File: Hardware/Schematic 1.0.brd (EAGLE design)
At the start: 119.4 x 63.5 mm, 58 parts, among them U2 ATMEGA328P-AU

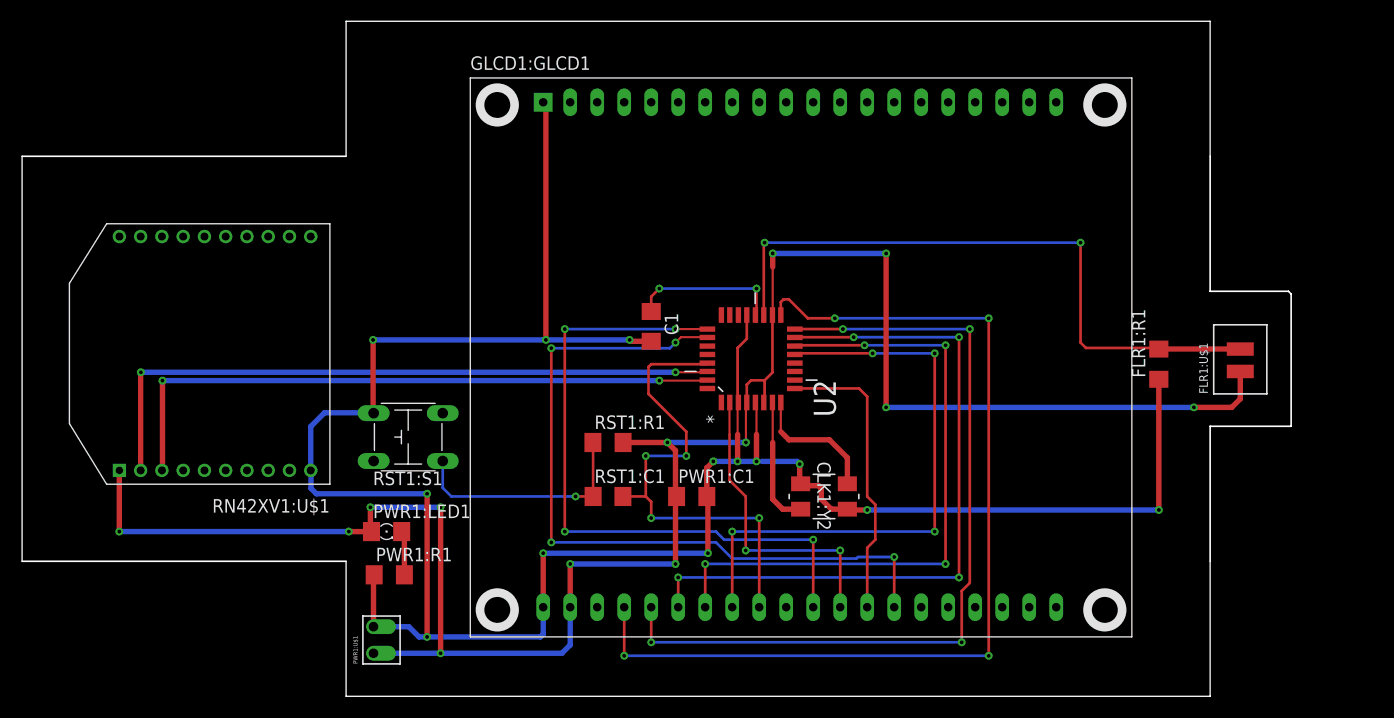
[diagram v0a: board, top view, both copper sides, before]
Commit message: Added Newest Hardware
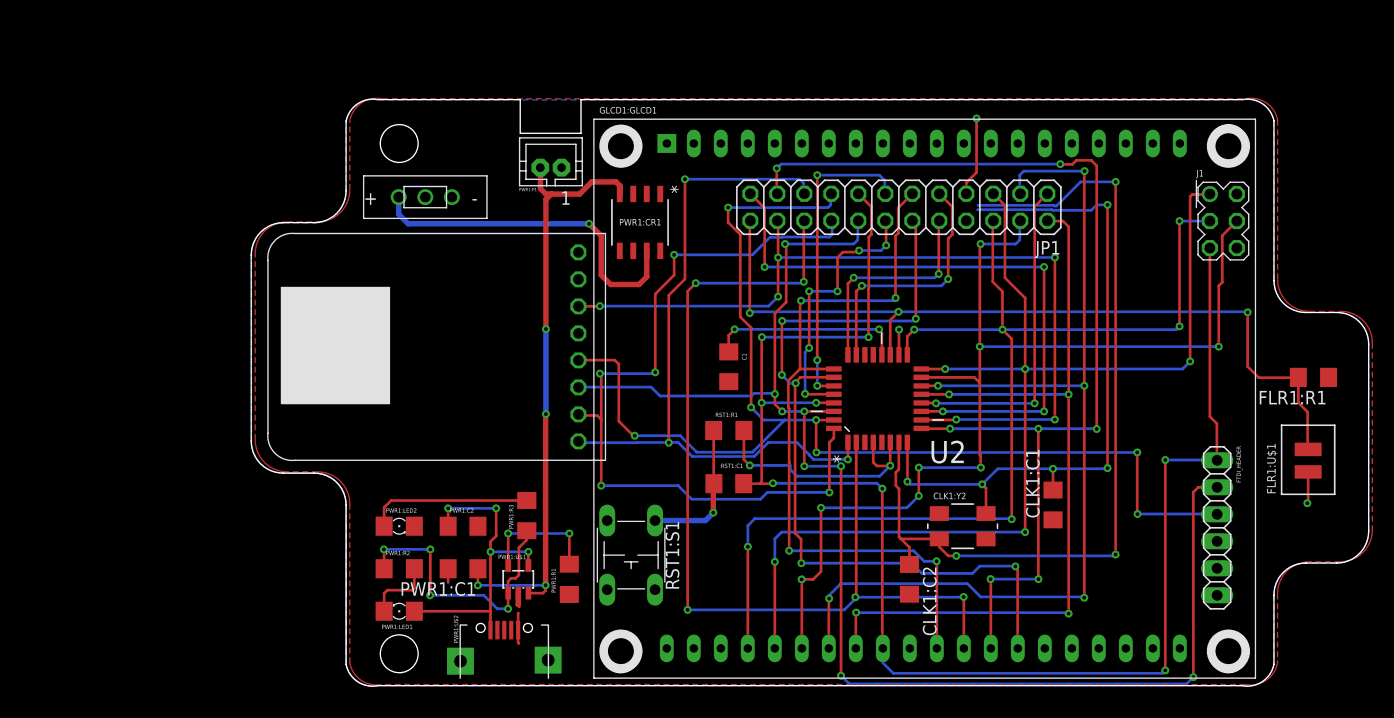
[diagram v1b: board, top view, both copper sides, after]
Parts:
- removed RN42XV1:U$1: RN42XV, RN42XV:RN42XV
- removed RN42XV1:U$10, RN42XV1:U$11, RN42XV1:U$12, RN42XV1:U$13, RN42XV1:U$14, RN42XV1:U$15, RN42XV1:U$16, RN42XV1:U$17, RN42XV1:U$2, RN42XV1:U$3, RN42XV1:U$4, RN42XV1:U$5, RN42XV1:U$6, RN42XV1:U$7, RN42XV1:U$8, RN42XV1:U$9: NC, Miscellaneous:NC
- added BLE-UART:U$1: BLE-UART, BLE-UART:BLE-UART
- added BLE-UART:U$2, PWR1:U$3, PWR1:U$4: NC, Miscellaneous:NC
- added CLK1:C1, CLK1:C2: 22pF, rcl:C1206
- added FTDI_HEADER: (no value), pinhead:1X06
- added J1: AVR-ISP-6PINAVR-ISP-6PIN-SMALL-SILK, avr-isp:AVR-ISP-6PIN-SMAILL-SILK
- added JP1: (no value), pinhead:2X12
- added PWR1:C2: 0.1uF, rcl:C1206
- added PWR1:CR1: LD1117D33CTR, LD1117 SMD:SO-8
- added PWR1:LED2: (no value), led:1206
- added PWR1:P1: (no value), jst-ph:JST-PH2
- added PWR1:R2, PWR1:R3: 470, resistor:R1206
- added PWR1:U$2: MICRO-USB, microusb:MICRO-USB
- added PWR1:U$5: EG1218-PWR-SW, EG1218-PWR-SW:EG1218-PWR-SW
- PWR1:C1: device resistor:R1206 -> rcl:C1206
- PWR1:R1: value 10k -> 2k
- PWR1:U$1: value JST-XH-F -> MCP73831; device ATBTLC1000-MR110CA:JST-XH-F -> mcp73831:SOT23-5L
- moved GLCD1:U$2 104.7 mm to (11.4, -8.89)
- moved GLCD1:U$3 104.7 mm to (11.4, -10.2)
- moved GLCD1:U$4 104.7 mm to (11.4, -11.4)
- moved GLCD1:U$1 104.7 mm to (11.4, -7.62)
- moved RST1:S1 23.7 mm to (26.8, 13.3), turned to 270 degrees
- moved PWR1:C1 22.6 mm to (11.0, 12.0), turned to 180 degrees
- moved PWR1:R1 16.9 mm to (21.0, 11.0), turned to 90 degrees
- moved FLR1:R1 14.6 mm to (91.0, 30.0), turned to 180 degrees
- moved PWR1:U$1 13.7 mm to (16.2, 11.0), turned to 0 degrees
- moved CLK1:Y2 13.3 mm to (58.0, 16.0)
- moved U2 12.5 mm to (50.0, 28.0)
- moved GLCD1:GLCD1 12.3 mm to (23.3, 1.71)
- moved RST1:C1 11.4 mm to (36.0, 20.0)
- moved RST1:R1 11.4 mm to (36.0, 25.0)
- moved FLR1:U$1 11.4 mm to (93.0, 19.0)
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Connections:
- new net 1/PD3/BLE_MOD: BLE-UART:U$1.1, JP1.19, U2.1
- new net 10/PD6/BLE_RTS: BLE-UART:U$1.6, JP1.22, U2.10
- new net 32/PD2/BLE_CTS: BLE-UART:U$1.2, JP1.18, U2.32
- new net N$10: J1.VCC
- new net PB0: JP1.1, U2.12
- new net PC0: JP1.9, U2.23
- new net PC1: JP1.10, U2.24
- new net PC4: JP1.13, U2.27
- new net PC5: JP1.14, U2.28
- new net PD7: JP1.23, U2.11
- new net PWR1:N$2: PWR1:LED1.C, PWR1:R2.2
- new net PWR1:N$3: PWR1:R2.1, PWR1:R3.1, PWR1:U$1.1
- new net PWR1:N$4: PWR1:LED2.A, PWR1:R3.2
- new net PWR1:N$5: PWR1:R1.2, PWR1:U$1.5
- new net PWR1:N$6: PWR1:CR1.7, PWR1:U$5.1
- new net PWR1:NS10: PWR1:C1.1, PWR1:CR1.4, PWR1:P1.2, PWR1:U$1.3
- net 13/PB1/LCD_C/!D: now also JP1.2
- net 14/PB2/!LCD_CS: now also JP1.3
- net 15/PB3/MOSI: now also J1.MOSI, JP1.4
- net 16/PB4/MISO: now also J1.MISO, JP1.5
- net 17/PB5/SCK: now also J1.SCK, JP1.6
- net 19/ADC6: now also JP1.24
- net 2/PD4/LCD_X+: now also JP1.20
- net 25/PC2/LCD_Y+: now also JP1.11
- net 26/PC3/LCD_X-: now also JP1.12
- net 29/PC6/!RESET: now also FTDI_HEADER.1, J1.RESET, JP1.15
- net 7/PB6/XTAL1: now also CLK1:C2.1
- net 8/PB7/XTAL2: now also CLK1:C1.2
- net 9/PD5/LCD_Y-: now also JP1.21
- net ATRXD_BLTXD: now also BLE-UART:U$1.3, FTDI_HEADER.2, JP1.16; no longer RN42XV1:U$1.2
- net ATTXD_BLRXD: now also BLE-UART:U$1.4, FTDI_HEADER.3, JP1.17; no longer RN42XV1:U$1.3
- net GND: now also BLE-UART:U$1.7, CLK1:C1.1, CLK1:C2.2, FTDI_HEADER.5, FTDI_HEADER.6, J1.GND, JP1.8, PWR1:C2.2, PWR1:CR1.1, PWR1:LED2.C, PWR1:P1.1, PWR1:U$1.2, PWR1:U$2.5, PWR1:U$2.GND1, PWR1:U$2.GND2, PWR1:U$5.3; no longer PWR1:U$1.GND, RN42XV1:U$1.10
- net PWR1:N$1: now also PWR1:C2.1, PWR1:LED1.A, PWR1:U$1.4, PWR1:U$2.1; no longer PWR1:LED1.C, PWR1:R1.2
- net VCC: now also BLE-UART:U$1.5, FTDI_HEADER.4, JP1.7, PWR1:U$5.2; no longer PWR1:C1.1, PWR1:LED1.A, PWR1:U$1.VCC, RN42XV1:U$1.1
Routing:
- net GND: track 223.4 -> 5.56 mm, vias 13 -> 0
- net VCC: track 195.0 -> 36.5 mm, vias 13 -> 5
- net 29/PC6/!RESET: track 46.1 -> 146.5 mm, vias 4 -> 8
- net 10/PD6/BLE_RTS: track 0.00 -> 80.2 mm, vias 0 -> 6
- net 32/PD2/BLE_CTS: track 0.00 -> 75.4 mm, vias 0 -> 5
- net 9/PD5/LCD_Y-: track 27.6 -> 99.5 mm, vias 0 -> 7
- net 7/PB6/XTAL1: track 12.1 -> 82.4 mm, vias 0 -> 3
- net ATRXD_BLTXD: track 62.6 -> 131.0 mm, vias 2 -> 8
- net 1/PD3/BLE_MOD: track 0.00 -> 66.6 mm, vias 0 -> 3
- net 2/PD4/LCD_X+: track 28.8 -> 93.0 mm, vias 2 -> 5
- net PD7: track 0.00 -> 58.9 mm, vias 0 -> 4
- net PWR1:NS10: track 0.00 -> 58.3 mm, vias 0 -> 4
- net ATTXD_BLRXD: track 59.8 -> 112.7 mm, vias 2 -> 7
- net 8/PB7/XTAL2: track 12.5 -> 65.4 mm, vias 0 -> 5
- net 15/PB3/MOSI: track 67.3 -> 100.4 mm, vias 4 -> 8
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- added copper zone on layer 1, net GND
- added copper zone on layer 16, net VCC
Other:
- board size 119.4 x 63.5 mm -> 105.1 x 55.2 mm
- board text added: "Funded by Trenton Evans UNL ECEN Capstone Team 4: SGS Rev. 2 - Aidan Colling - Michael Goberling - Jacob Pilakowski"
